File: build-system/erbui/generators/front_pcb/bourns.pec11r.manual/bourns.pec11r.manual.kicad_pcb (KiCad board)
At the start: 2 copper layers, 1 part

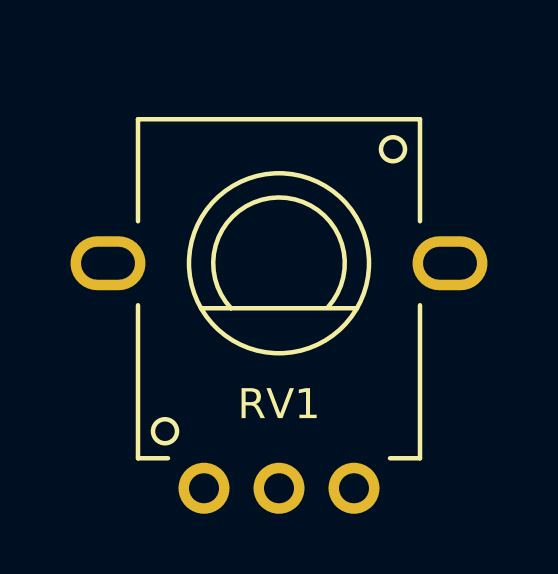
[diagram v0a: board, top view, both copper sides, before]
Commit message: fixup! Add encoder
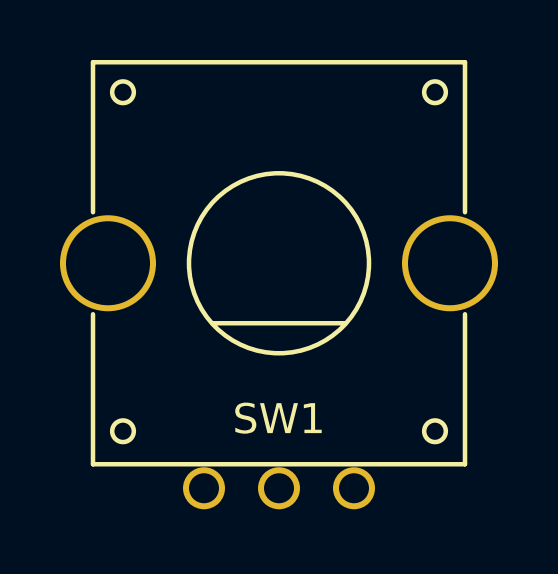
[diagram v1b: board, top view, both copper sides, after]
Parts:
- removed RV1: 100k, Potentiometer_Thonk:AlphaPot9ShaftD
- added SW1: RotaryEncoder, local:PEC11R-4220F-N0024, F.Cu at (0.00, 0.00)
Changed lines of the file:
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@@
   (net 0 "")
   (net 1 "+3V3")
-  (net 2 "GND")
+  (net 2 "Pin1")
   (net 3 "Pin0")
-  (footprint "Potentiometer_Thonk:AlphaPot9ShaftD" locked (layer "F.Cu")
+  (footprint "local:PEC11R-4220F-N0024" locked (layer "F.Cu")
     (at 0 0)
+    (property "Description" "ROTARY ENCODER MECHANICAL 24PPR")
+    (property "Device" "Encoder")
+    (property "Dist" "DigiKey")
+    (property "DistLink" "https://www.digikey.de/en/products/detail/bourns-inc/PEC11R-4220F-N0024/4699220")
+    (property "DistPartNumber" "PEC11R-4220F-N0024-ND")
+    (property "Place" "No")
+    (property "Sheetfile" "bourns.pec11r.manual.kicad_sch")
+    (property "Sheetname" "")
     (attr through_hole)
-    (fp_text reference "RV1" (at 0 4.7) (layer "F.SilkS")
+    (fp_text reference "SW1" (at 0 5.2 unlocked) (layer "F.SilkS")
       (effects (font (size 1 1) (thickness 0.15)))
     )
-    (fp_text value "100k" (at 0 10.1) (layer "F.Fab")
+    (fp_text value "RotaryEncoder" (at 0 -7.7 unlocked) (layer "F.Fab")
       (effects (font (size 1 1) (thickness 0.15)))
     )
-    (fp_line (start -4.7 -4.8) (end 4.7 -4.8) (layer "F.SilkS") (width 0.15))
-    (fp_line (start -4.7 -4.8) (end -4.7 -1.4) (layer "F.SilkS") (width 0.15))
-    (fp_line (start -2.6 1.5) (end 2.6 1.5) (layer "F.SilkS") (width 0.15))
-    (fp_line (start 4.7 1.4) (end 4.7 6.5) (layer "F.SilkS") (width 0.15))
-    (fp_line (start -4.7 1.4) (end -4.7 6.5) (layer "F.SilkS") (width 0.15))
-    (fp_line (start -4.7 6.5) (end -3.7 6.5) (layer "F.SilkS") (width 0.15))
-    (fp_line (start 3.7 6.5) (end 4.7 6.5) (layer "F.SilkS") (width 0.15))
-    (fp_line (start 4.7 -4.8) (end 4.7 -1.4) (layer "F.SilkS") (width 0.15))
-    (fp_arc (start -1.6 1.5) (mid -0.024972 -2.193029) (end 1.633741 1.463178) (layer "F.SilkS") (width 0.15))
-    (fp_circle (center 3.8 -3.8) (end 4.2 -3.8) (layer "F.SilkS") (width 0.15) (fill none))
-    (fp_circle (center -3.8 5.6) (end -4.2 5.6) (layer "F.SilkS") (width 0.15) (fill none))
+    (fp_line (start 6.2 6.7) (end 6.2 1.7) (layer "F.SilkS") (width 0.15))
+    (fp_line (start -6.2 -6.7) (end -6.2 -1.7) (layer "F.SilkS") (width 0.15))
+    (fp_line (start -6.2 6.7) (end -6.2 1.7) (layer "F.SilkS") (width 0.15))
+    (fp_line (start -2.2 2) (end 2.2 2) (layer "F.SilkS") (width 0.15))
+    (fp_line (start 6.2 -6.7) (end 6.2 -1.7) (layer "F.SilkS") (width 0.15))
+    (fp_line (start -6.2 -6.7) (end 6.2 -6.7) (layer "F.SilkS") (width 0.15))
+    (fp_line (start -6.2 6.7) (end 6.2 6.7) (layer "F.SilkS") (width 0.15))
+    (fp_circle (center 5.2 -5.7) (end 5.560555 -5.7) (layer "F.SilkS") (width 0.15) (fill none))
     (fp_circle (center 0 0) (end 3 0) (layer "F.SilkS") (width 0.15) (fill none))
-    (pad "" thru_hole oval locked (at -5.7 0) (size 2.5 1.8) (drill oval 1.8 1.1) (layers *.Cu *.Mask))
-    (pad "" thru_hole oval locked (at 5.7 0) (size 2.5 1.8) (drill oval 1.8 1.1) (layers *.Cu *.Mask))
-    (pad "1" thru_hole oval locked (at -2.5 7.5) (size 1.7 1.7) (drill 1) (layers *.Cu *.Mask)
-      (net 2 "GND"))
-    (pad "2" thru_hole oval locked (at 0 7.5) (size 1.7 1.7) (drill 1) (layers *.Cu *.Mask)
-      (net 3 "Pin0"))
-    (pad "3" thru_hole oval locked (at 2.5 7.5) (size 1.7 1.7) (drill 1) (layers *.Cu *.Mask)
-      (net 1 "+3V3"))
+    (fp_circle (center -5.2 -5.7) (end -5 -5.4) (layer "F.SilkS") (width 0.15) (fill none))
+    (fp_circle (center -5.2 5.6) (end -5 5.9) (layer "F.SilkS") (width 0.15) (fill none))
+    (fp_circle (center 5.2 5.6) (end 5.560555 5.6) (layer "F.SilkS") (width 0.15) (fill none))
+    (pad "" thru_hole circle locked (at -5.7 0) (size 3.2 3.2) (drill 2.8) (layers *.Cu *.Mask))
+    (pad "" thru_hole circle locked (at 5.7 0) (size 3.2 3.2) (drill 2.8) (layers *.Cu *.Mask))
+    (pad "A" thru_hole circle locked (at -2.5 7.5) (size 1.4 1.4) (drill 1) (layers *.Cu *.Mask)
+      (net 3 "Pin0") (pinfunction "A") (pintype "passive"))
+    (pad "B" thru_hole circle locked (at 2.5 7.5) (size 1.4 1.4) (drill 1) (layers *.Cu *.Mask)
+      (net 2 "Pin1") (pinfunction "B") (pintype "passive"))
+    (pad "C" thru_hole circle locked (at 0 7.5) (size 1.4 1.4) (drill 1) (layers *.Cu *.Mask)
+      (net 1 "+3V3") (pinfunction "C") (pintype "passive"))
   )
   (gr_circle (center 0 0) (end 3.75 0) (layer "Eco1.User") (width 0.12) (fill none))
